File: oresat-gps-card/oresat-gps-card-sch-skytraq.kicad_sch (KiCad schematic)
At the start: 11 parts, among them U23 ORION-B16

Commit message: BOM Update
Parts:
- C75: DIS (none) -> DigiKey; DPN (none) -> 399-6856-1-ND; MFR (none) -> KEMET; MPN (none) -> C0603C104K5RACAUTO
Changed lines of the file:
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@@
 			)
 		)
-		(property "Datasheet" ""
+		(property "Datasheet" "https://search.kemet.com/download/specsheet/C0603C104K5RACAUTO"
 			(at 205.74 93.98 0)
 			(hide yes)
@@
 			)
 		)
-		(property "Description" "Unpolarized capacitor"
+		(property "Description" "0.1 µF ±10% 50V Ceramic Capacitor X7R 0603 (1608 Metric)"
 			(at 205.74 93.98 0)
 			(hide yes)
+			(show_name no)
+			(do_not_autoplace no)
+			(effects
+				(font
+					(size 1.27 1.27)
+				)
+			)
+		)
+		(property "DIS" "DigiKey"
+			(at 205.74 93.98 0)
+			(hide yes)
+			(show_name no)
+			(do_not_autoplace no)
+			(effects
+				(font
+					(size 1.27 1.27)
+				)
+			)
+		)
+		(property "DPN" "399-6856-1-ND"
+			(at 205.74 93.98 0)
+			(hide yes)
+			(show_name no)
+			(do_not_autoplace no)
+			(effects
+				(font
+					(size 1.27 1.27)
+				)
+			)
+		)
+		(property "MFR" "KEMET"
+			(at 205.74 93.98 0)
+			(hide yes)
+			(show_name no)
+			(do_not_autoplace no)
+			(effects
+				(font
+					(size 1.27 1.27)
+				)
+			)
+		)
+		(property "MPN" "C0603C104K5RACAUTO"
+			(at 205.74 93.98 0)
+			(hide yes)

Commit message: Large BOM changes for v1.2, no changes to PCB
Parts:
- TP20, TP23, TP24: value 1x01 -> Test-Point; now left out of the parts list
- U23: DIS (none) -> N/A; DPN (none) -> N/A; MFR (none) -> Skytraq; MPN (none) -> ORION B16
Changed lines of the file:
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@@
 		(body_style 1)
 		(exclude_from_sim no)
-		(in_bom yes)
+		(in_bom no)
 		(on_board yes)
 		(in_pos_files yes)
@@
 			)
 		)
-		(property "Value" "1x01"
+		(property "Value" "Test-Point"
 			(at 175.26 144.78 0)
 			(hide yes)
@@
 		)
 		(property "Footprint" "oresat-misc:TestPoint-0.75mm-th"
-			(at 175.26 144.78 0)
+			(at 175.26 137.16 0)
 			(hide yes)
 			(show_name no)
@@
 		)
 		(property "Datasheet" ""
-			(at 175.26 144.78 0)
-			(hide yes)
-			(show_name no)
-			(do_not_autoplace no)
-			(effects
-				(font
-					(size 1.27 1.27)
-				)
-			)
-		)
-		(property "Description" ""
+			(at 175.26 147.32 0)
+			(hide yes)
+			(show_name no)
+			(do_not_autoplace no)
+			(effects
+				(font
+					(size 1.27 1.27)
+				)
+			)
+		)
+		(property "Description" "0.75 mm TH test point; good for scope probes and jumpers"
 			(at 175.26 147.32 0)
 			(hide yes)
@@
 		(body_style 1)
 		(exclude_from_sim no)
-		(in_bom yes)
+		(in_bom no)
 		(on_board yes)
 		(in_pos_files yes)
@@
 			)
 		)
-		(property "Value" "1x01"
+		(property "Value" "Test-Point"
 			(at 175.26 142.24 0)
 			(hide yes)
@@
 		)
 		(property "Footprint" "oresat-misc:TestPoint-0.75mm-th"
-			(at 175.26 142.24 0)
+			(at 175.26 134.62 0)
 			(hide yes)
 			(show_name no)
@@
 		)
 		(property "Datasheet" ""
-			(at 175.26 142.24 0)
-			(hide yes)
-			(show_name no)
-			(do_not_autoplace no)
-			(effects
-				(font
-					(size 1.27 1.27)
-				)
-			)
-		)
-		(property "Description" ""
+			(at 175.26 144.78 0)
+			(hide yes)
+			(show_name no)
+			(do_not_autoplace no)
+			(effects
+				(font
+					(size 1.27 1.27)
+				)
+			)
+		)
+		(property "Description" "0.75 mm TH test point; good for scope probes and jumpers"
 			(at 175.26 144.78 0)
 			(hide yes)
@@
 		(body_style 1)
 		(exclude_from_sim no)
-		(in_bom yes)
+		(in_bom no)
 		(on_board yes)
 		(in_pos_files yes)
@@
 			)
 		)
-		(property "Value" "1x01"
+		(property "Value" "Test-Point"
 			(at 236.22 124.46 0)
 			(hide yes)
@@
 		)
 		(property "Footprint" "oresat-misc:TestPoint-0.75mm-th"
-			(at 236.22 124.46 0)
+			(at 236.22 116.84 0)
 			(hide yes)
 			(show_name no)
@@
 		)
 		(property "Datasheet" ""
-			(at 236.22 124.46 0)
-			(hide yes)
-			(show_name no)
-			(do_not_autoplace no)
-			(effects
-				(font
-					(size 1.27 1.27)
-				)
-			)
-		)
-		(property "Description" ""
+			(at 236.22 127 0)
+			(hide yes)
+			(show_name no)
+			(do_not_autoplace no)
+			(effects
+				(font
+					(size 1.27 1.27)
+				)
+			)
+		)
+		(property "Description" "0.75 mm TH test point; good for scope probes and jumpers"
 			(at 236.22 127 0)
 			(hide yes)
@@
 			)
 		)
-		(property "Description" ""
+		(property "Description" "LEO capable GNSS receiver"
 			(at 162.56 135.89 0)
 			(hide yes)
 			(show_name no)
+			(do_not_autoplace no)
+			(effects
+				(font
+					(size 1.27 1.27)
+				)
+			)
+		)
+		(property "DIS" "N/A"
+			(at 215.9 134.62 0)
+			(hide yes)
+			(show_name no)
+			(do_not_autoplace no)
+			(effects
+				(font
+					(size 1.27 1.27)
+				)
+			)
+		)
+		(property "DPN" "N/A"
+			(at 215.9 134.62 0)
+			(hide yes)
+			(show_name no)
+			(do_not_autoplace no)
+			(effects
+				(font
+					(size 1.27 1.27)
+				)
+			)
+		)
+		(property "MFR" "Skytraq"
+			(at 215.9 134.62 0)
+			(hide yes)
+			(show_name no)
+			(do_not_autoplace no)
+			(effects
+				(font
+					(size 1.27 1.27)
+				)
+			)
+		)
+		(property "MPN" "ORION B16"
+			(at 215.9 134.62 0)
+			(hide yes)
+			(show_name no)

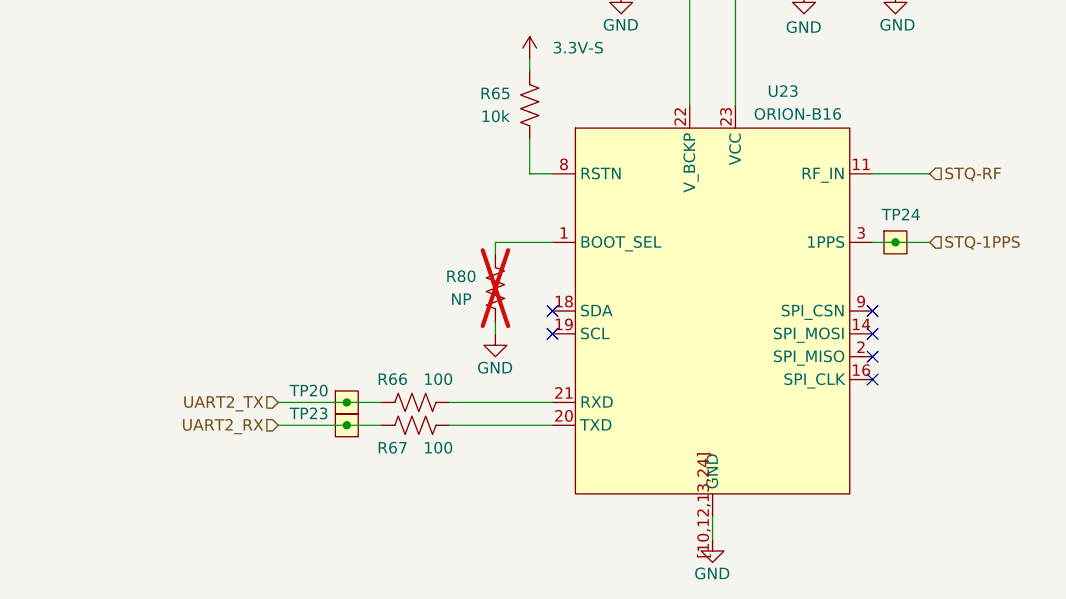
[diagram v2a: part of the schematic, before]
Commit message: Upped to v1.3.
Fixed backward EEPROM programming pin, fixed potential boot error with missing PMIC connections, fixed some power domain issues.
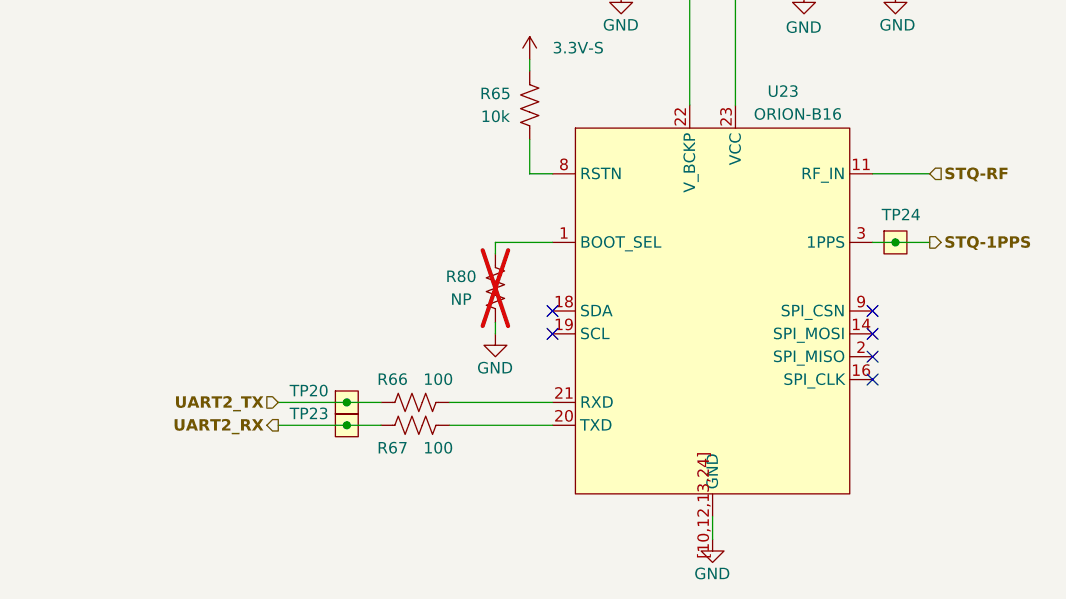
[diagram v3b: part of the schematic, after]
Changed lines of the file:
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@@
 	(title_block
 		(title "OreSat GPS Card")
-		(date "2026-07-06")
-		(rev "1.2")
+		(date "2026-09-17")
+		(rev "1.3")
 		(company "Portland State Aerospace Society")
 	)
@@
 			(font
 				(size 1.27 1.27)
+				(thickness 0.254)
+				(bold yes)
 			)
 			(justify left)
@@
 	)
 	(hierarchical_label "STQ-1PPS"
-		(shape input)
+		(shape output)
 		(at 240.03 127 0)
 		(effects
 			(font
 				(size 1.27 1.27)
+				(thickness 0.254)
+				(bold yes)
 			)
 			(justify left)
@@
 	)
 	(hierarchical_label "UART2_RX"
-		(shape input)
+		(shape output)
 		(at 167.64 147.32 180)
 		(effects
 			(font
 				(size 1.27 1.27)
+				(thickness 0.254)
+				(bold yes)
 			)
 			(justify right)
@@
 			(font
 				(size 1.27 1.27)
+				(thickness 0.254)
+				(bold yes)
 			)
 			(justify right)
